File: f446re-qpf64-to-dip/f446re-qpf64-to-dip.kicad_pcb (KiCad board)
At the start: 2 copper layers, 26.7 x 82.6 mm, 4 parts, among them J1 Conn_01x32_Pin, J2 Conn_01x32_Pin, U1 STM32F446RETx

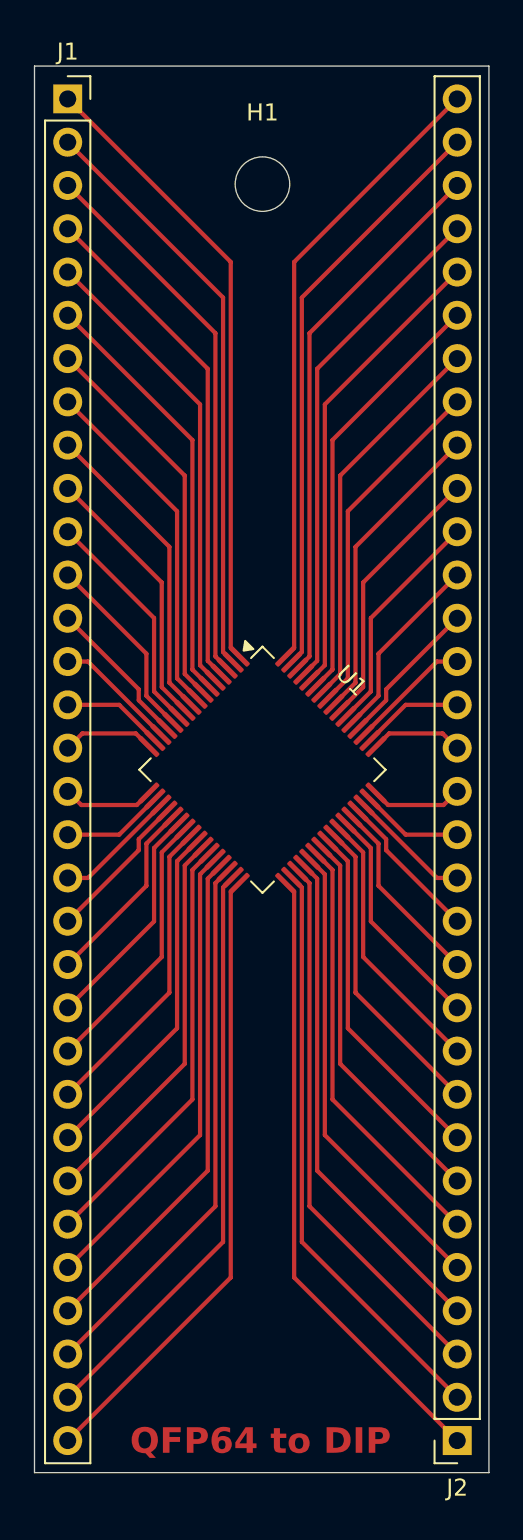
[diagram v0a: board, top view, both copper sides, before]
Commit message: hoge
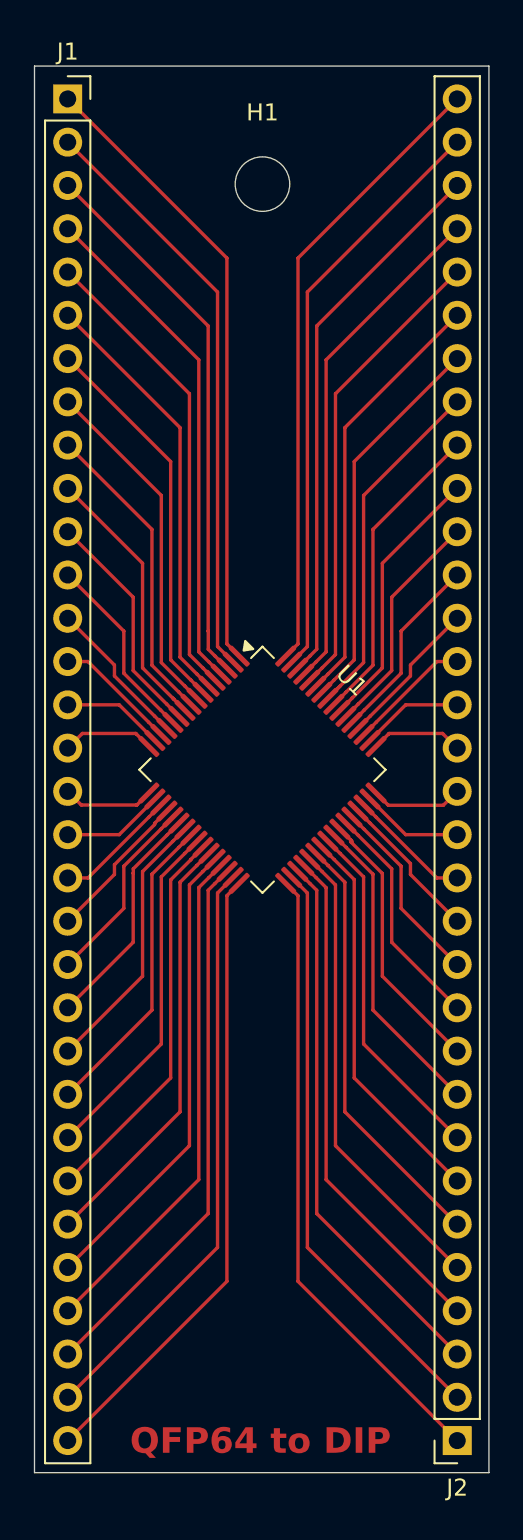
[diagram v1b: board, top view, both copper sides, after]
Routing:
- net Net-(J2-Pin_25): track 20.5 -> 21.6 mm
